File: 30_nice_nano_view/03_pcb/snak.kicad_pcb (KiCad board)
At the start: 2 copper layers, 114 x 99 mm, 114 parts

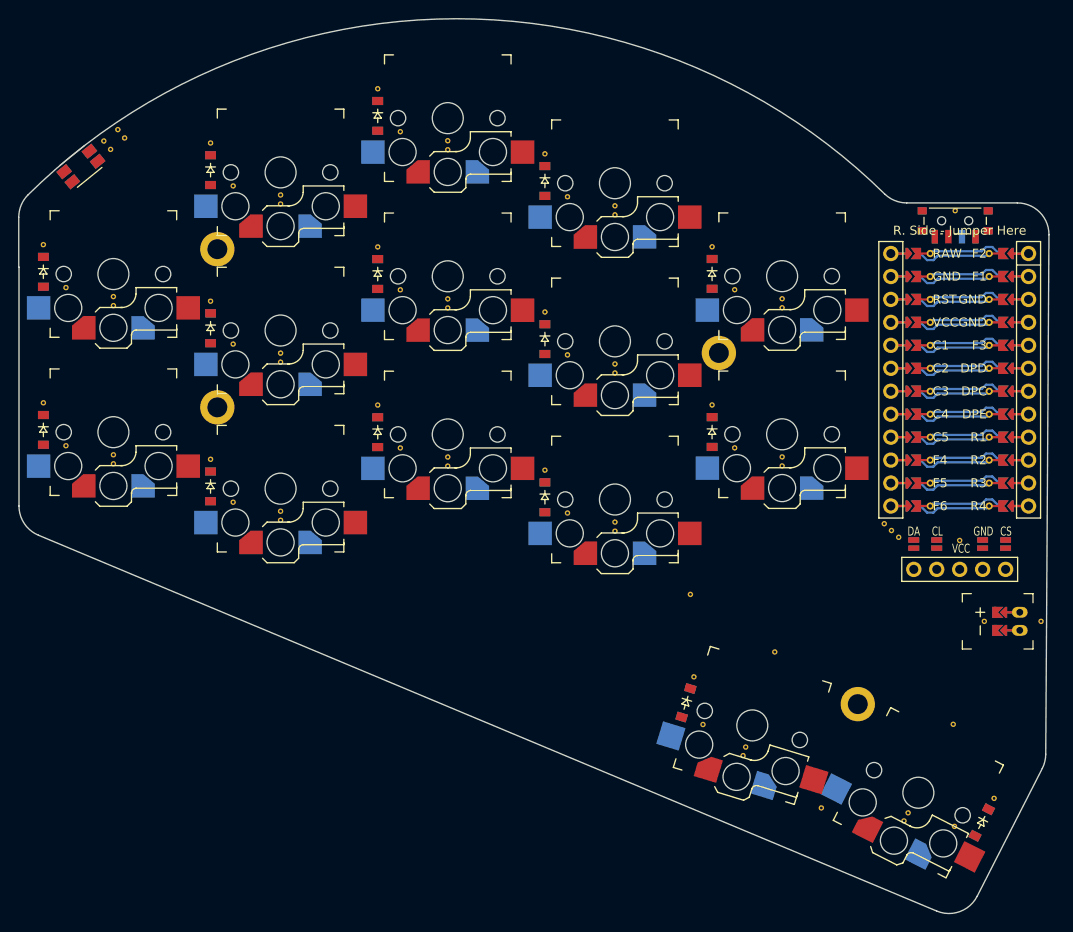
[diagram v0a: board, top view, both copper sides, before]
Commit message: update
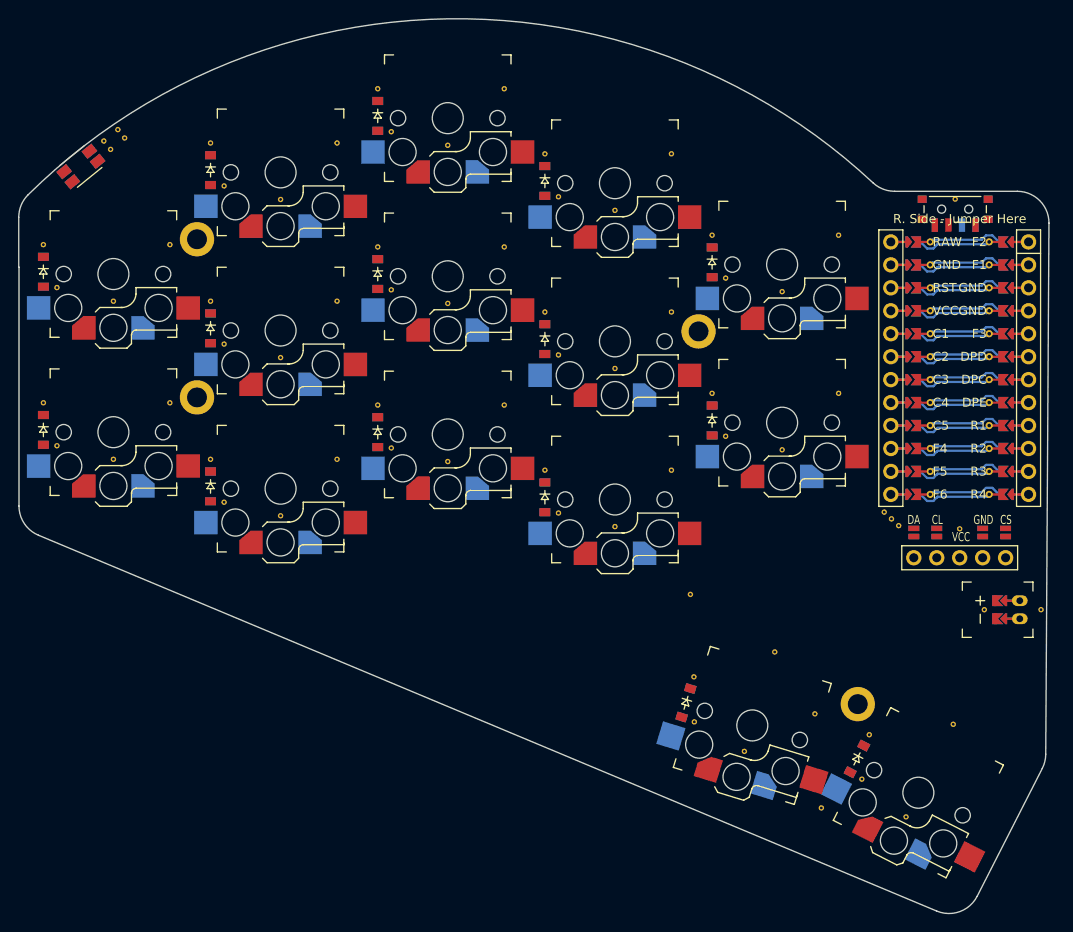
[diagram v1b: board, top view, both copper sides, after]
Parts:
- removed the REF** at (166.2, 79.5)
- removed the REF** at (166.2, 62.0)
- removed the REF** at (197.5, 123.0)
- removed the REF** at (94.8, 84.0)
- removed the REF** at (94.8, 66.5)
- removed the REF** at (113.2, 90.2)
- removed the REF** at (113.2, 72.8)
- removed the REF** at (113.2, 55.2)
- removed the REF** at (131.8, 84.2)
- removed the REF** at (131.8, 66.8)
- removed the REF** at (131.8, 49.2)
- removed the REF** at (150.2, 91.5)
- removed the REF** at (150.2, 74.0)
- removed the REF** at (150.2, 56.5)
- removed the REF** at (168.8, 84.2)
- removed the REF** at (168.8, 66.7)
- removed the REF** at (165.2, 114.8)
- removed the REF** at (193.1, 126.1)
- removed the REF** at (100.0, 85.0)
- removed the REF** at (100.0, 67.5)
- removed the REF** at (118.5, 91.2)
- removed the REF** at (118.5, 73.8)
- removed the REF** at (118.5, 56.2)
- removed the REF** at (137.0, 85.2)
- removed the REF** at (137.0, 67.8)
- removed the REF** at (137.0, 50.2)
- removed the REF** at (155.5, 92.5)
- removed the REF** at (155.5, 75.0)
- removed the REF** at (155.5, 57.5)
- removed the REF** at (174.0, 85.2)
- removed the REF** at (174.0, 67.7)
- removed the REF** at (170.0, 117.3)
- removed the REF** at (187.9, 124.6)
- removed the REF** at (100.0, 86.0)
- removed the REF** at (100.0, 68.5)
- removed the REF** at (118.5, 92.2)
- removed the REF** at (118.5, 74.8)
- removed the REF** at (118.5, 57.2)
- removed the REF** at (137.0, 86.2)
- removed the REF** at (137.0, 68.8)
- removed the REF** at (137.0, 51.2)
- removed the REF** at (155.5, 93.5)
- removed the REF** at (155.5, 76.0)
- removed the REF** at (155.5, 58.5)
- removed the REF** at (174.0, 86.2)
- removed the REF** at (174.0, 68.7)
- removed the REF** at (169.7, 118.3)
- removed the REF** at (187.5, 125.5)
- removed the REF** at (186.9, 94.1)
- removed the REF** at (186.1, 93.4)
- removed the REF** at (185.3, 92.6)
- removed the REF** at (193.7, 94.5)
- removed the REF** at (193.2, 58.0)
- removed the REF** at (196.4, 103.4)
- removed the REF** at (202.7, 103.4)
- added REF**: VIA-0.6mm, VIA-0.6mm, F.Cu at (166.2, 78.2)
- added REF**: VIA-0.6mm, VIA-0.6mm, F.Cu at (166.2, 60.7)
- added REF**: VIA-0.6mm, VIA-0.6mm, F.Cu at (183.6, 116.0)
- added REF**: VIA-0.6mm, VIA-0.6mm, F.Cu at (93.8, 84.0)
- added REF**: VIA-0.6mm, VIA-0.6mm, F.Cu at (93.8, 66.5)
- added REF**: VIA-0.6mm, VIA-0.6mm, F.Cu at (112.2, 90.2)
- added REF**: VIA-0.6mm, VIA-0.6mm, F.Cu at (112.2, 72.8)
- added REF**: VIA-0.6mm, VIA-0.6mm, F.Cu at (112.2, 55.2)
- added REF**: VIA-0.6mm, VIA-0.6mm, F.Cu at (130.8, 84.2)
- added REF**: VIA-0.6mm, VIA-0.6mm, F.Cu at (130.8, 66.8)
- added REF**: VIA-0.6mm, VIA-0.6mm, F.Cu at (130.8, 49.2)
- added REF**: VIA-0.6mm, VIA-0.6mm, F.Cu at (149.2, 91.5)
- added REF**: VIA-0.6mm, VIA-0.6mm, F.Cu at (149.2, 74.0)
- added REF**: VIA-0.6mm, VIA-0.6mm, F.Cu at (149.2, 56.5)
- added REF**: VIA-0.6mm, VIA-0.6mm, F.Cu at (167.8, 83.0)
- added REF**: VIA-0.6mm, VIA-0.6mm, F.Cu at (167.8, 65.5)
- added REF**: VIA-0.6mm, VIA-0.6mm, F.Cu at (164.3, 114.6)
- added REF**: VIA-0.6mm, VIA-0.6mm, F.Cu at (182.8, 120.9)
- added REF**: VIA-0.6mm, VIA-0.6mm, F.Cu at (106.2, 79.2)
- added REF**: VIA-0.6mm, VIA-0.6mm, F.Cu at (106.2, 61.8)
- added REF**: VIA-0.6mm, VIA-0.6mm, F.Cu at (124.8, 85.5)
- added REF**: VIA-0.6mm, VIA-0.6mm, F.Cu at (124.8, 68.0)
- added REF**: VIA-0.6mm, VIA-0.6mm, F.Cu at (124.8, 50.5)
- added REF**: VIA-0.6mm, VIA-0.6mm, F.Cu at (143.2, 79.5)
- added REF**: VIA-0.6mm, VIA-0.6mm, F.Cu at (143.2, 62.0)
- added REF**: VIA-0.6mm, VIA-0.6mm, F.Cu at (143.2, 44.5)
- added REF**: VIA-0.6mm, VIA-0.6mm, F.Cu at (161.8, 86.7)
- added REF**: VIA-0.6mm, VIA-0.6mm, F.Cu at (161.8, 69.2)
- added REF**: VIA-0.6mm, VIA-0.6mm, F.Cu at (161.8, 51.7)
- added REF**: VIA-0.6mm, VIA-0.6mm, F.Cu at (180.2, 78.2)
- added REF**: VIA-0.6mm, VIA-0.6mm, F.Cu at (180.2, 60.7)
- added REF**: VIA-0.6mm, VIA-0.6mm, F.Cu at (177.6, 113.7)
- added REF**: VIA-0.6mm, VIA-0.6mm, F.Cu at (100.0, 85.5)
- added REF**: VIA-0.6mm, VIA-0.6mm, F.Cu at (100.0, 68.0)
- added REF**: VIA-0.6mm, VIA-0.6mm, F.Cu at (118.5, 91.8)
- added REF**: VIA-0.6mm, VIA-0.6mm, F.Cu at (118.5, 74.2)
- added REF**: VIA-0.6mm, VIA-0.6mm, F.Cu at (118.5, 56.8)
- added REF**: VIA-0.6mm, VIA-0.6mm, F.Cu at (137.0, 85.8)
- added REF**: VIA-0.6mm, VIA-0.6mm, F.Cu at (137.0, 68.2)
- added REF**: VIA-0.6mm, VIA-0.6mm, F.Cu at (137.0, 50.8)
- added REF**: VIA-0.6mm, VIA-0.6mm, F.Cu at (155.5, 93.0)
- added REF**: VIA-0.6mm, VIA-0.6mm, F.Cu at (155.5, 75.5)
- added REF**: VIA-0.6mm, VIA-0.6mm, F.Cu at (155.5, 58.0)
- added REF**: VIA-0.6mm, VIA-0.6mm, F.Cu at (174.0, 84.5)
- added REF**: VIA-0.6mm, VIA-0.6mm, F.Cu at (174.0, 67.0)
- added REF**: VIA-0.6mm, VIA-0.6mm, F.Cu at (169.8, 117.8)
- added REF**: VIA-0.6mm, VIA-0.6mm, F.Cu at (187.7, 125.1)
- added REF**: VIA-0.6mm, VIA-0.6mm, F.Cu at (186.9, 92.8)
- added REF**: VIA-0.6mm, VIA-0.6mm, F.Cu at (186.1, 92.1)
- added REF**: VIA-0.6mm, VIA-0.6mm, F.Cu at (185.3, 91.3)
- added REF**: VIA-0.6mm, VIA-0.6mm, F.Cu at (193.7, 93.2)
- added REF**: VIA-0.6mm, VIA-0.6mm, F.Cu at (193.2, 56.7)
- added REF**: VIA-0.6mm, VIA-0.6mm, F.Cu at (196.4, 102.1)
- added REF**: VIA-0.6mm, VIA-0.6mm, F.Cu at (202.7, 102.1)
- moved D15 15.5 mm to (182.3, 118.7)
- moved H3 3.28 mm to (164.8, 71.4)
- moved H1 2.50 mm to (109.2, 61.1)
- moved H2 2.50 mm to (109.2, 78.7)
- moved D12 1.29 mm to (166.2, 81.2)
- moved D13 1.29 mm to (166.2, 63.7)
- moved DISP1 1.29 mm to (193.7, 79.7)
- moved JST1 1.29 mm to (200.3, 102.1)
- moved MCU1 1.29 mm to (193.7, 74.1)
- moved S12 1.29 mm to (174.0, 81.5)
- moved S13 1.29 mm to (174.0, 64.0)
- moved SW1 1.29 mm to (193.2, 57.8)
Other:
- outline, holes or cut-outs redrawn

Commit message: update
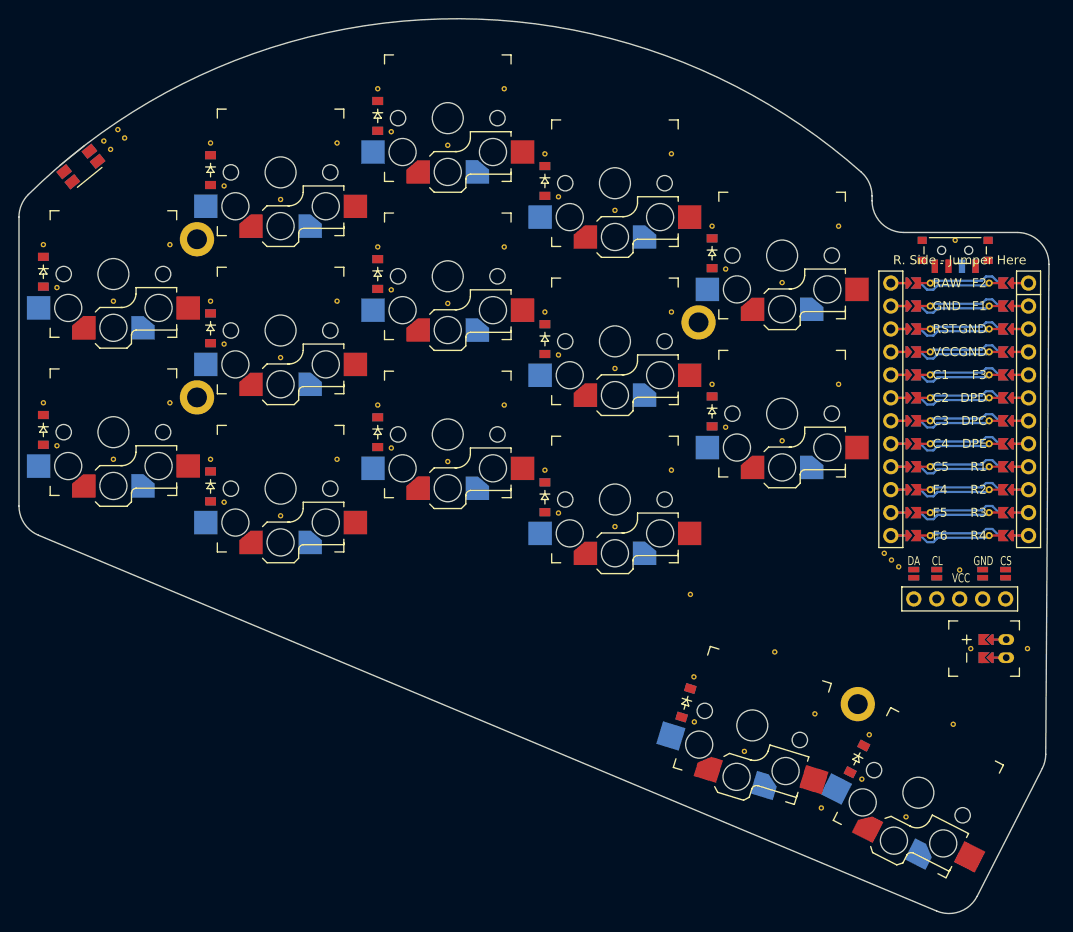
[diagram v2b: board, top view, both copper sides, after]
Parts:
- removed the REF** at (166.2, 78.2)
- removed the REF** at (166.2, 60.7)
- removed the REF** at (167.8, 83.0)
- removed the REF** at (167.8, 65.5)
- removed the REF** at (180.2, 78.2)
- removed the REF** at (180.2, 60.7)
- removed the REF** at (174.0, 84.5)
- removed the REF** at (174.0, 67.0)
- removed the REF** at (186.9, 92.8)
- removed the REF** at (186.1, 92.1)
- removed the REF** at (185.3, 91.3)
- removed the REF** at (193.7, 93.2)
- removed the REF** at (193.2, 56.7)
- removed the REF** at (196.4, 102.1)
- removed the REF** at (202.7, 102.1)
- added REF**: VIA-0.6mm, VIA-0.6mm, F.Cu at (166.2, 77.2)
- added REF**: VIA-0.6mm, VIA-0.6mm, F.Cu at (166.2, 59.7)
- added REF**: VIA-0.6mm, VIA-0.6mm, F.Cu at (167.8, 82.0)
- added REF**: VIA-0.6mm, VIA-0.6mm, F.Cu at (167.8, 64.5)
- added REF**: VIA-0.6mm, VIA-0.6mm, F.Cu at (180.2, 77.2)
- added REF**: VIA-0.6mm, VIA-0.6mm, F.Cu at (180.2, 59.7)
- added REF**: VIA-0.6mm, VIA-0.6mm, F.Cu at (174.0, 83.5)
- added REF**: VIA-0.6mm, VIA-0.6mm, F.Cu at (174.0, 66.0)
- added REF**: VIA-0.6mm, VIA-0.6mm, F.Cu at (186.9, 97.4)
- added REF**: VIA-0.6mm, VIA-0.6mm, F.Cu at (186.1, 96.7)
- added REF**: VIA-0.6mm, VIA-0.6mm, F.Cu at (185.3, 95.9)
- added REF**: VIA-0.6mm, VIA-0.6mm, F.Cu at (193.7, 97.8)
- added REF**: VIA-0.6mm, VIA-0.6mm, F.Cu at (193.2, 61.3)
- added REF**: VIA-0.6mm, VIA-0.6mm, F.Cu at (194.9, 106.5)
- added REF**: VIA-0.6mm, VIA-0.6mm, F.Cu at (201.2, 106.5)
- moved JST1 4.56 mm to (198.8, 106.5)
- moved DISP1 4.55 mm to (193.7, 84.2)
- moved MCU1 4.55 mm to (193.7, 78.7)
- moved SW1 4.55 mm to (193.2, 62.4)
- moved D12 1.00 mm to (166.2, 80.2)
- moved D13 1.00 mm to (166.2, 62.7)
- moved H3 1.00 mm to (164.8, 70.4)
- moved S12 1.00 mm to (174.0, 80.5)
- moved S13 1.00 mm to (174.0, 63.0)
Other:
- outline, holes or cut-outs redrawn
